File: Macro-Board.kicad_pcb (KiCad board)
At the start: 2 copper layers, 152.4 x 133.3 mm, 62 parts, among them J1 esp32row1, J2 esp32row1, K1 KEYSW, K10 KEYSW, K11 KEYSW, K12 KEYSW, K13 KEYSW, K14 KEYSW, K15 KEYSW, K16 KEYSW, K17 KEYSW, K18 KEYSW, K19 KEYSW, K2 KEYSW, K20 KEYSW, K21 KEYSW, K22 KEYSW, K23 KEYSW, K24 KEYSW, K25 KEYSW, K27 KEYSW, K28 KEYSW, K29 KEYSW, K3 KEYSW, K30 KEYSW, K4 KEYSW, K5 KEYSW, K6 KEYSW, K7 KEYSW, K8 KEYSW, K9 KEYSW, SW26 RotaryEncoder_Alps_EC11E-Swit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

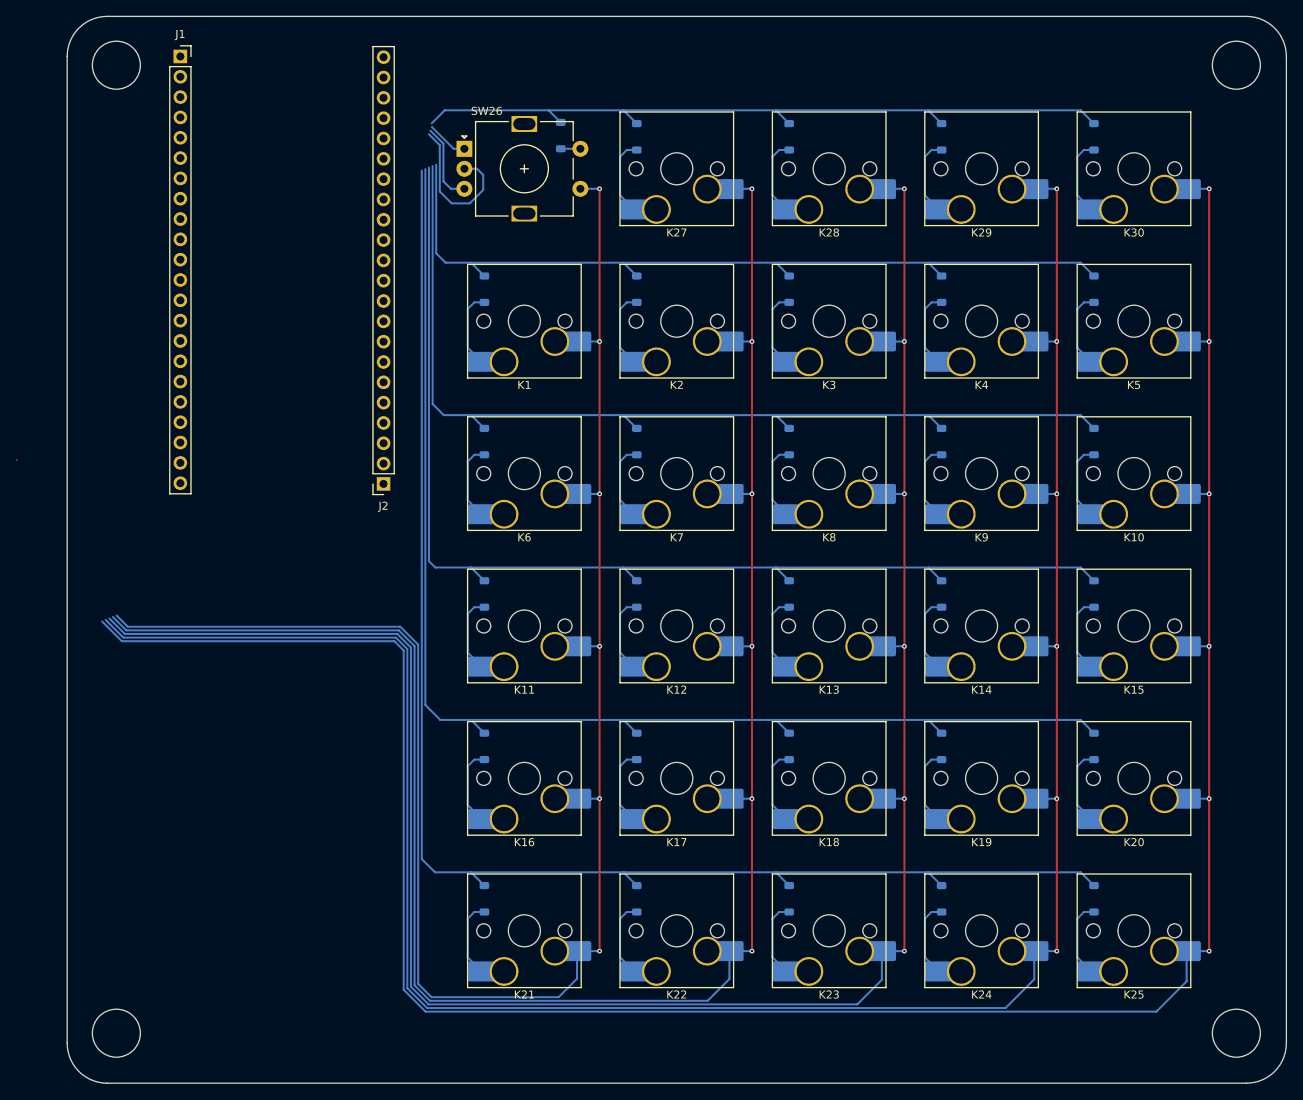
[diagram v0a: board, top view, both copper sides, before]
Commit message: Idfk
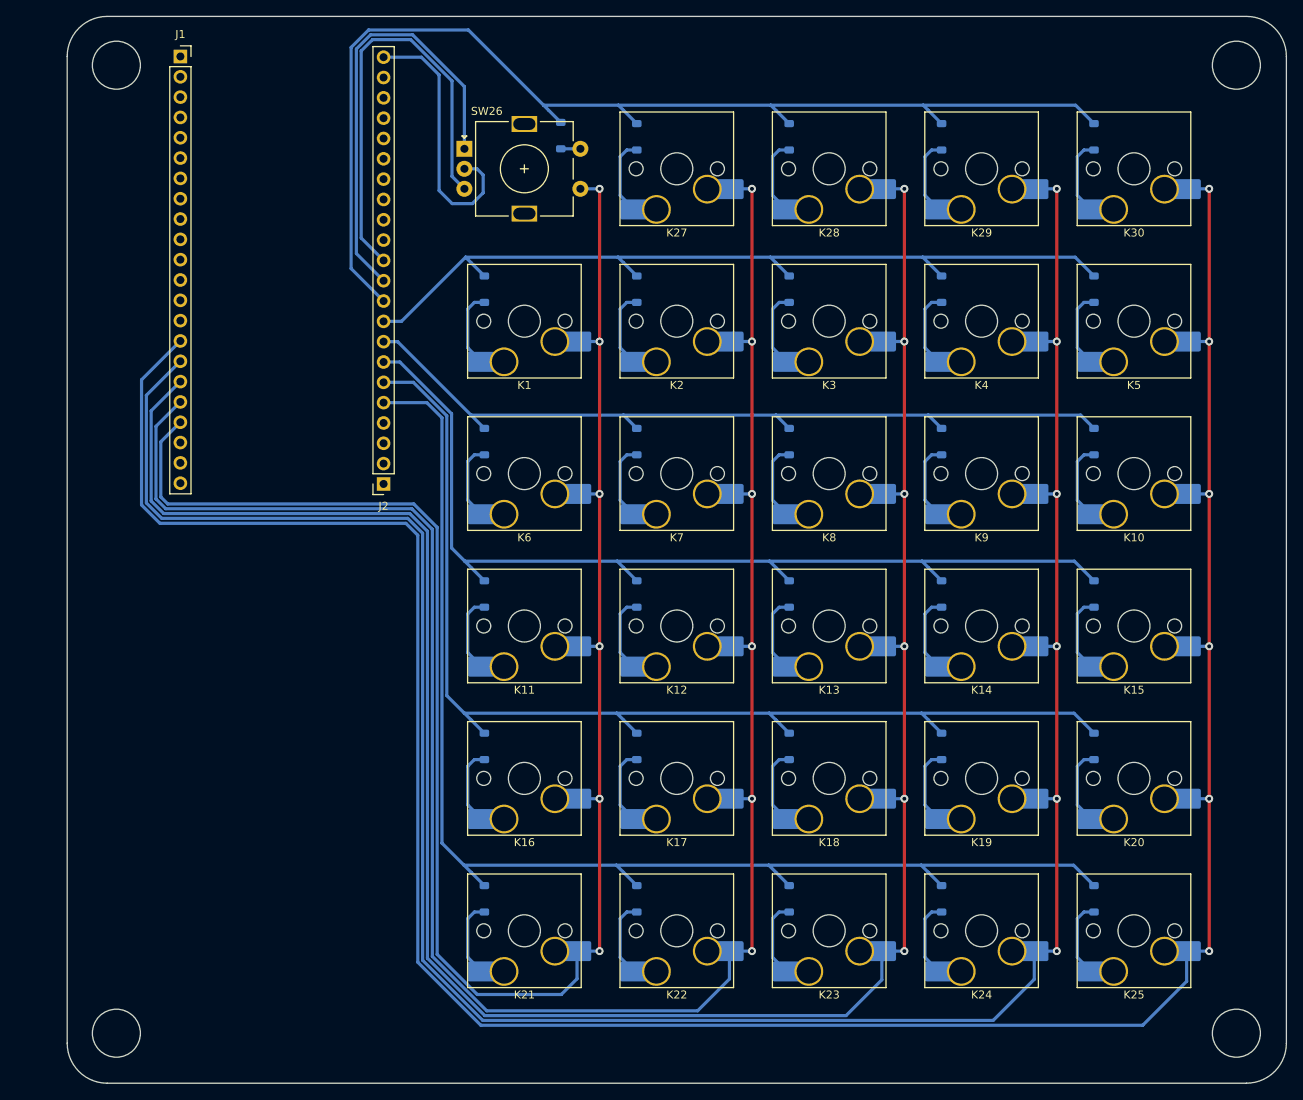
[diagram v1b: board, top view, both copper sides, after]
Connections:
- D1 pad 1: /GPIO42 -> /GPIO16
- D10 pad 1: /GPIO41 -> /GPIO15
- D11 pad 1: /GPIO40 -> /GPIO07
- D12 pad 1: /GPIO40 -> /GPIO07
- D13 pad 1: /GPIO40 -> /GPIO07
- D14 pad 1: /GPIO40 -> /GPIO07
- D15 pad 1: /GPIO40 -> /GPIO07
- D16 pad 1: /GPIO39 -> /GPIO06
- D17 pad 1: /GPIO39 -> /GPIO06
- D18 pad 1: /GPIO39 -> /GPIO06
- D19 pad 1: /GPIO39 -> /GPIO06
- D2 pad 1: /GPIO42 -> /GPIO16
- D20 pad 1: /GPIO39 -> /GPIO06
- D21 pad 1: /GPIO38 -> /GPIO05
- D22 pad 1: /GPIO38 -> /GPIO05
- D23 pad 1: /GPIO38 -> /GPIO05
- D24 pad 1: /GPIO38 -> /GPIO05
- D25 pad 1: /GPIO38 -> /GPIO05
- D26 pad 1: /GPIO04 -> /GPIO17
- D27 pad 1: /GPIO04 -> /GPIO17
- D28 pad 1: /GPIO04 -> /GPIO17
- D29 pad 1: /GPIO04 -> /GPIO17
- D3 pad 1: /GPIO42 -> /GPIO16
- D30 pad 1: /GPIO04 -> /GPIO17
- D4 pad 1: /GPIO42 -> /GPIO16
- D5 pad 1: /GPIO42 -> /GPIO16
- D6 pad 1: /GPIO41 -> /GPIO15
- D7 pad 1: /GPIO41 -> /GPIO15
- D8 pad 1: /GPIO41 -> /GPIO15
- D9 pad 1: /GPIO41 -> /GPIO15
- J2 pad 10: /EncoderB -> /GPIO17
- J2 pad 11: /GPIO18 -> /EncoderA
- J2 pad 12: /GPIO08 -> /EncoderB
- J2 pad 9: /EncoderA -> /GPIO16
- K1 pad 1: /GPIO08 -> /GPIO01
- K10 pad 1: /GPIO05 -> /GPIO40
- K11 pad 1: /GPIO08 -> /GPIO01
- K12 pad 1: /GPIO15 -> /GPIO02
- K13 pad 1: /GPIO07 -> /GPIO42
- K14 pad 1: /GPIO06 -> /GPIO41
- K15 pad 1: /GPIO05 -> /GPIO40
- K16 pad 1: /GPIO08 -> /GPIO01
- K17 pad 1: /GPIO15 -> /GPIO02
- K18 pad 1: /GPIO07 -> /GPIO42
- K19 pad 1: /GPIO06 -> /GPIO41
- K2 pad 1: /GPIO15 -> /GPIO02
- K20 pad 1: /GPIO05 -> /GPIO40
- K21 pad 1: /GPIO08 -> /GPIO01
- K22 pad 1: /GPIO15 -> /GPIO02
- K23 pad 1: /GPIO07 -> /GPIO42
- K24 pad 1: /GPIO06 -> /GPIO41
- K25 pad 1: /GPIO05 -> /GPIO40
- K27 pad 1: /GPIO15 -> /GPIO02
- K28 pad 1: /GPIO07 -> /GPIO42
- K29 pad 1: /GPIO06 -> /GPIO41
- K3 pad 1: /GPIO07 -> /GPIO42
- K30 pad 1: /GPIO05 -> /GPIO40
- K4 pad 1: /GPIO06 -> /GPIO41
- K5 pad 1: /GPIO05 -> /GPIO40
- K6 pad 1: /GPIO08 -> /GPIO01
- K7 pad 1: /GPIO15 -> /GPIO02
- K8 pad 1: /GPIO07 -> /GPIO42
- K9 pad 1: /GPIO06 -> /GPIO41
- SW26 pad C: /GND4 -> /GND1
- SW26 pad S1: /GPIO08 -> /GPIO01
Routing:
- net /GPIO02: track 0.00 -> 259.7 mm, vias 0 -> 6
- net /GPIO01: track 0.00 -> 235.5 mm, vias 0 -> 6
- net /GPIO08: track 218.3 -> 0.00 mm, vias 6 -> 0
- net /GPIO40: track 142.7 -> 329.2 mm, vias 0 -> 6
- net /GPIO41: track 123.1 -> 305.9 mm, vias 0 -> 6
- net /GPIO38: track 180.8 -> 0.00 mm
- net /GPIO42: track 103.9 -> 282.9 mm, vias 0 -> 6
- net /GPIO39: track 161.4 -> 0.00 mm
- net /GPIO17: track 0.00 -> 144.8 mm
- net /GPIO05: track 297.7 -> 159.4 mm, vias 6 -> 0
- net /GPIO06: track 277.8 -> 141.6 mm, vias 6 -> 0
- net /GPIO15: track 238.2 -> 102.7 mm, vias 6 -> 0
- net /GPIO07: track 258.0 -> 123.8 mm, vias 6 -> 0
- net /GPIO16: track 0.00 -> 106.4 mm
- net /GPIO04: track 93.3 -> 0.00 mm
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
